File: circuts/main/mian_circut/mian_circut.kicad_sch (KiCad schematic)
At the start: 75 parts, among them J1 12v Power, J2 5v Power, J3 buzzer, J4 DE9_Plug, J5 metal detect, J6 Conn_02x04_Odd_Even, J7 302-S101, Q1 FDS4559, Q3 BC817, U1 ESP32-DEVKIT-V1, U3 ESP32-DEVKITC-32D, U4 78M05 SMD

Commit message: local_grib
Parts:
- J4: value DE9_Plug -> motor_con
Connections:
- net HVblock is gone; now on net HV: C3.1, D1.1 (K), D15.1 (A1), D2.K, F1.1, J4.1, J4.6
- net 12v: no longer C12.1, C13.1, C14.1, C15.1, C16.1, C17.1, C18.1, C19.1, R9.2
- net HV: now also C12.1, C13.1, C14.1, C15.1, C16.1, C17.1, C18.1, C19.1, R9.2
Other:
- moved on the sheet: C1, C28, C29, C3, D1, D12, D15, D16, D2, D3, D4, D8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

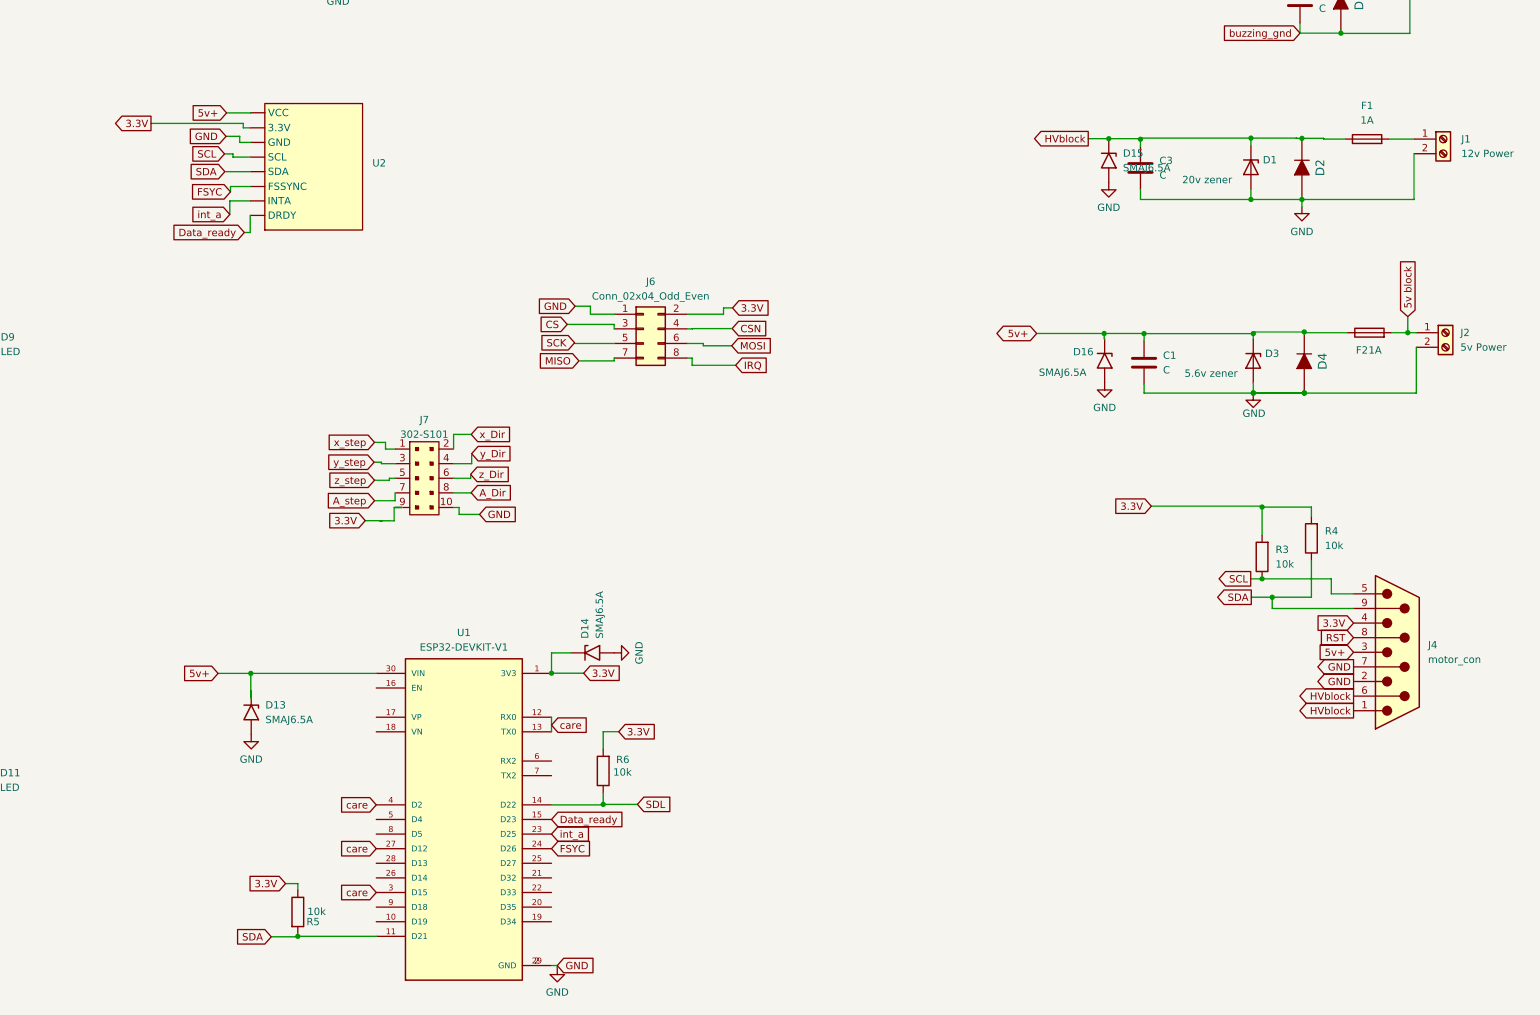
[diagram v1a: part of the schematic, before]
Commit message: compact ic int
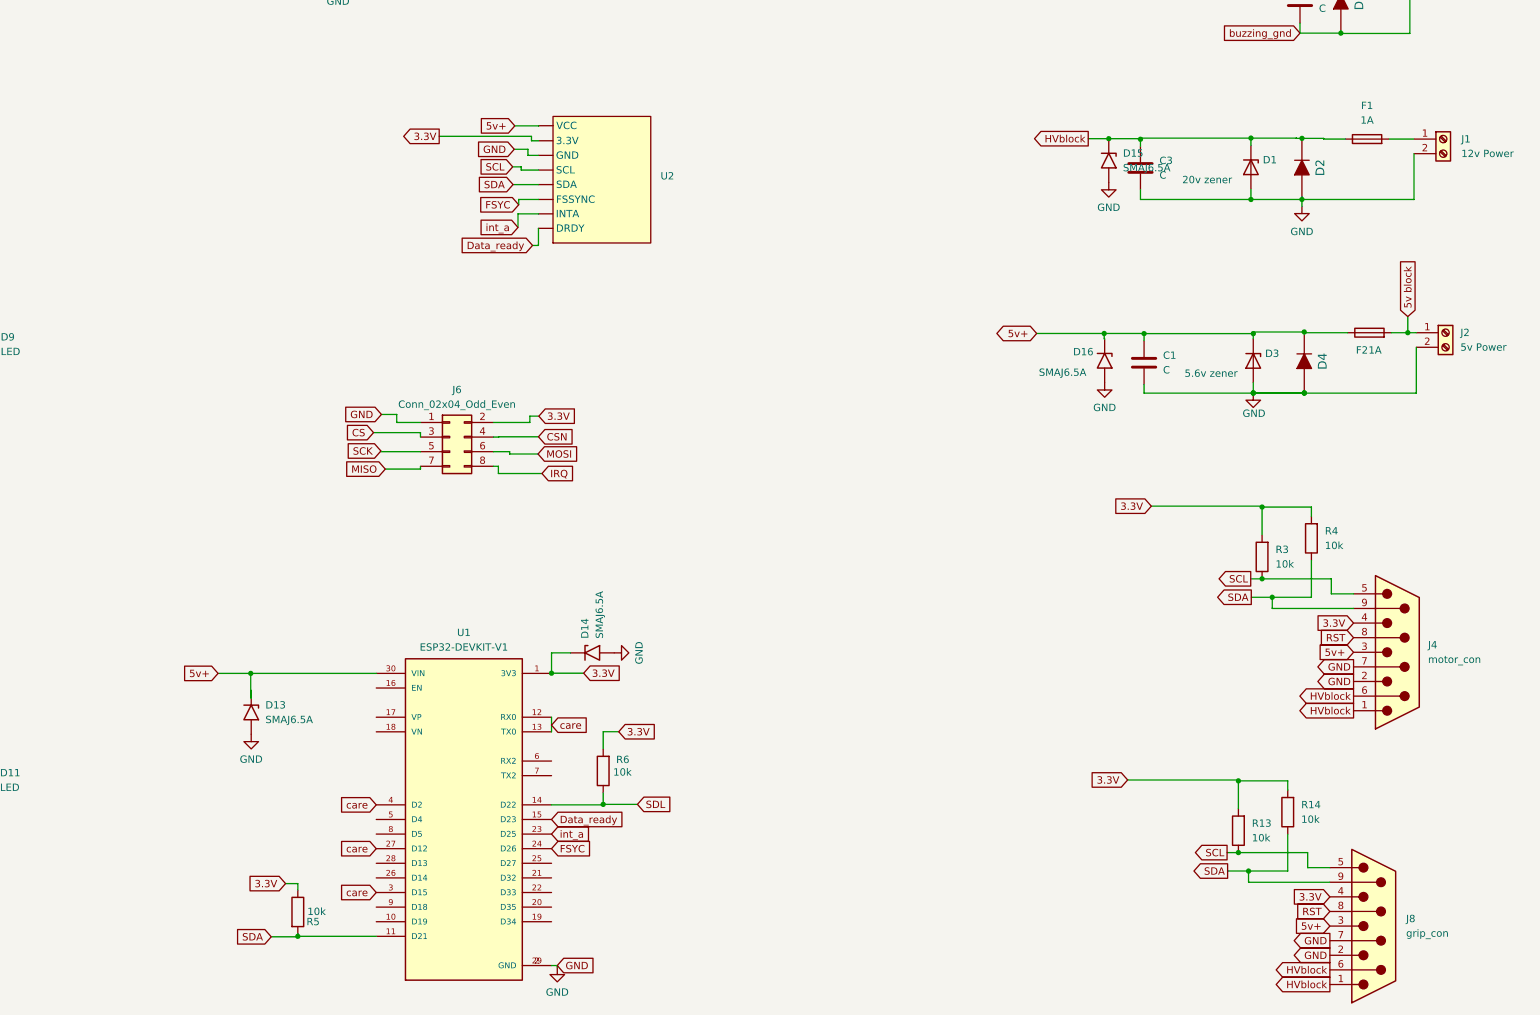
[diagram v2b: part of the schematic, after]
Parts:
- removed J7: 302-S101, digikey-footprints:PinHeader_2x5_P2.54mm_Drill1.2mm, symbol dk_Rectangular-Connectors-Headers-Male-Pins:302-S101
- added J8: grip_con, Connector_Dsub:DSUB-9_Male_Horizontal_P2.77x2.54mm_EdgePinOffset9.40mm, symbol Connector:DE9_Plug
- added R13, R14: 10k, Resistor_SMD:R_0805_2012Metric_Pad1.20x1.40mm_HandSolder, symbol Device:R
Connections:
- net 3.3V: now also J8.4, R13.2, R14.2
- net 5v+: now also J8.3
- net GND: now also J8.2, J8.7
- net HV: now also J8.1, J8.6
- net RST: now also J8.8
- net SCL: now also J8.5, R13.1
- net SDA: now also J8.9, R14.1
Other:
- moved on the sheet: J6, U2

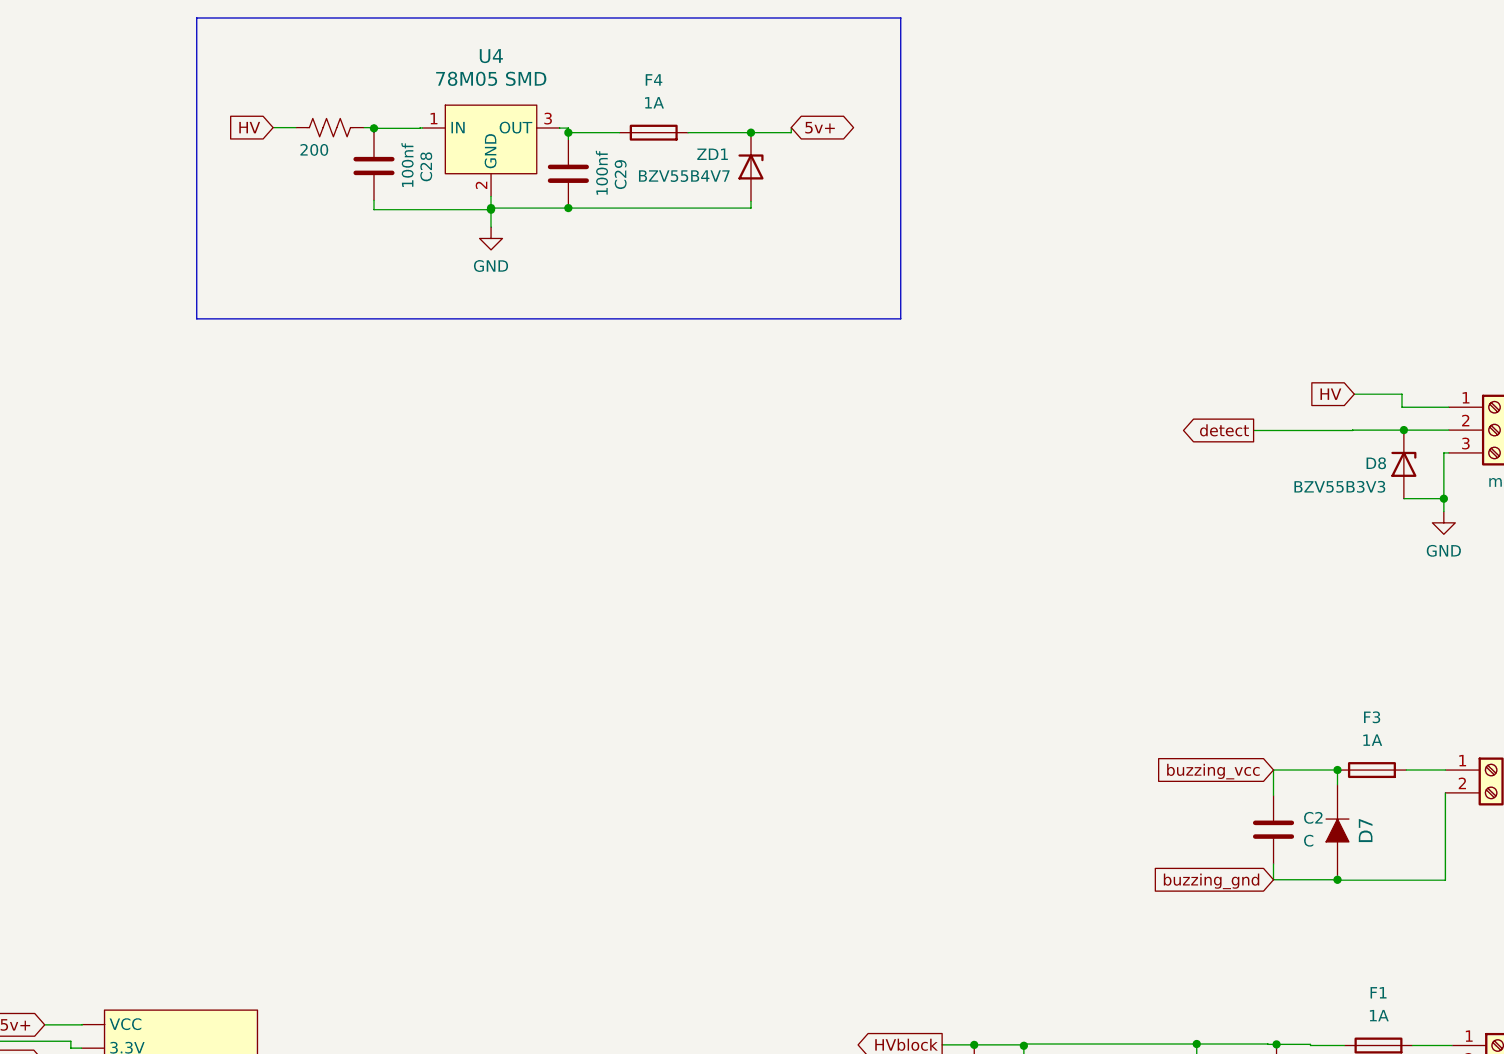
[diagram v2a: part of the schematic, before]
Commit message: last_touches
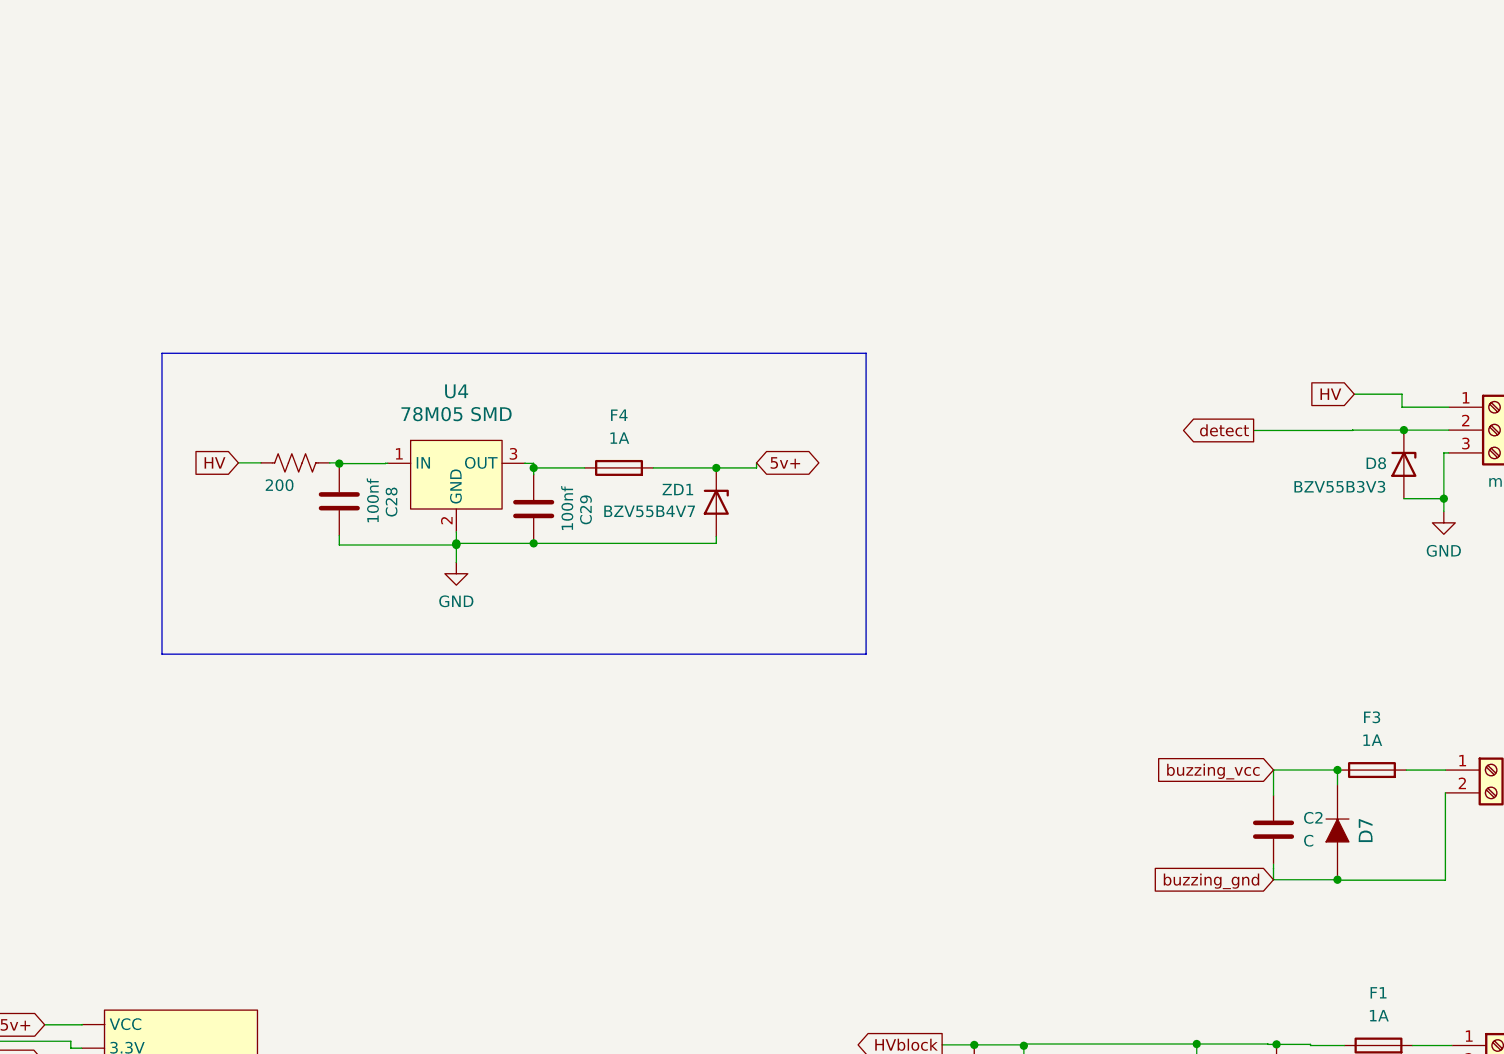
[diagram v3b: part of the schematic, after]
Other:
- moved on the sheet: C28, C29, F4, U4, ZD1
